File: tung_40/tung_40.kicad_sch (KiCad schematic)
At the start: 7 parts, among them J1 Conn_01x02_Male, J2 Conn_01x02_Male, SW1 GateronLP, SW5 SW_DIP_x03, U1 NRF52840-DONGLE

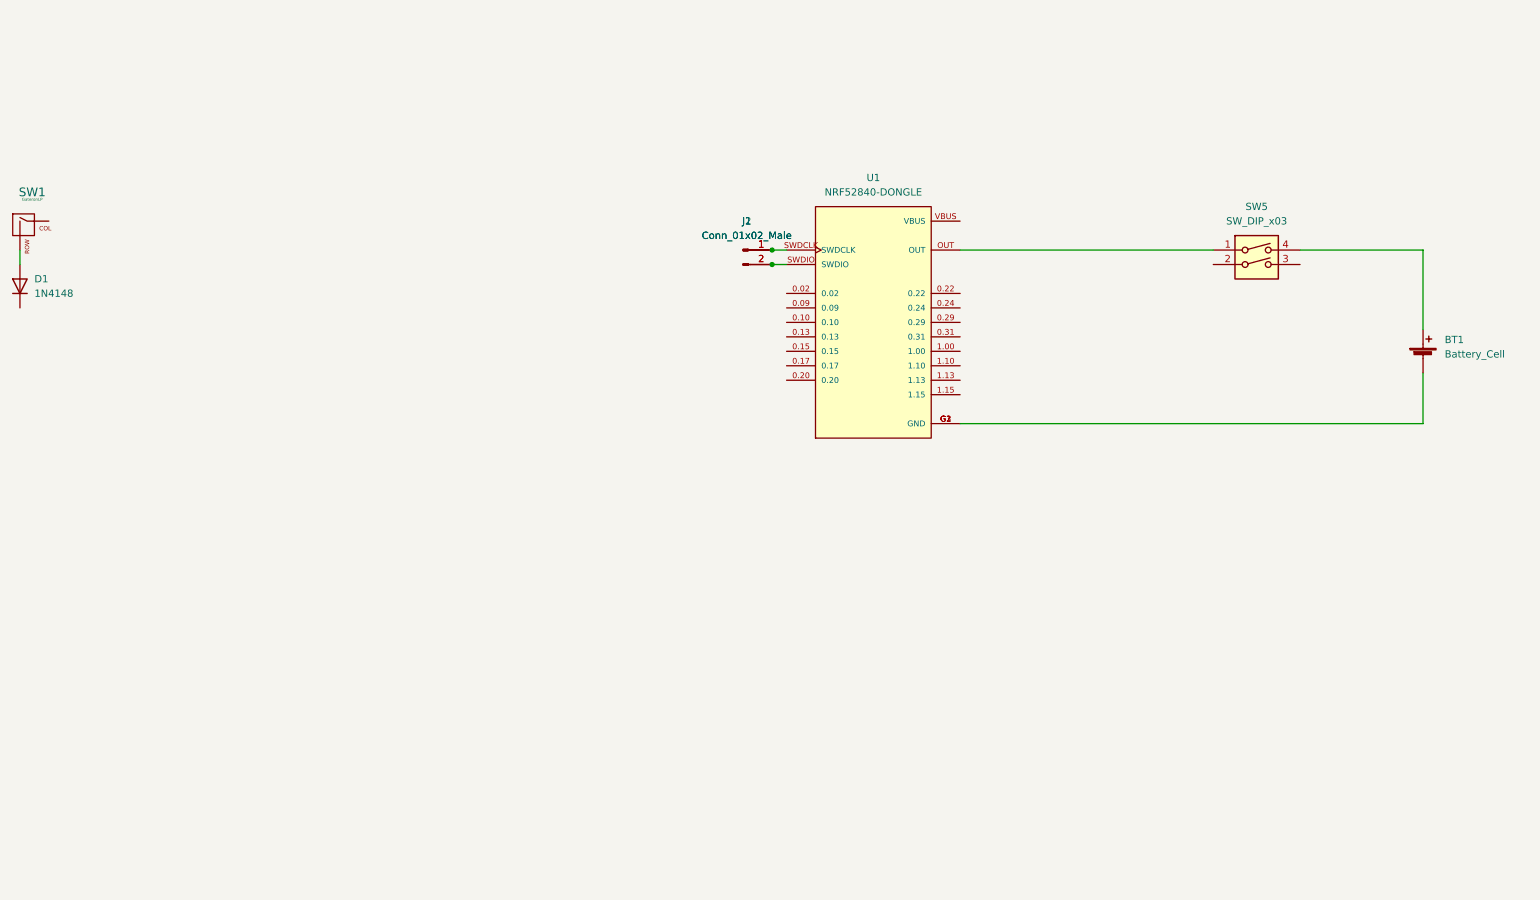
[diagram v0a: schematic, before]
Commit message: 48 keys in progress
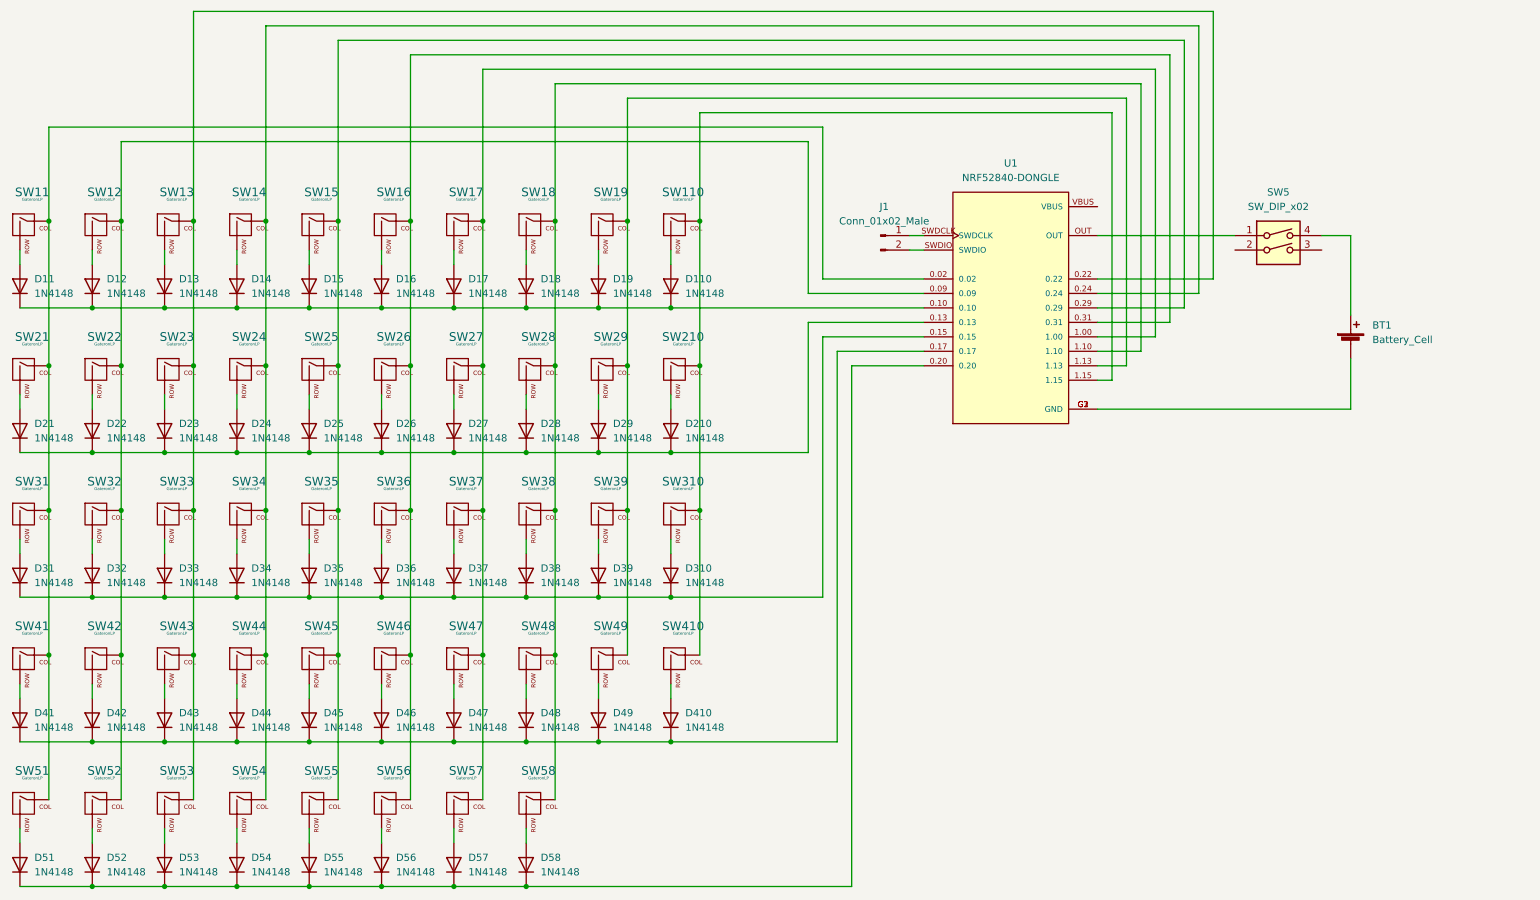
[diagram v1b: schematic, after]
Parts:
- removed J2: Conn_01x02_Male, Connector_PinHeader_2.54mm:PinHeader_1x02_P2.54mm_Vertical, symbol Connector:Conn_01x02_Male
- added D110, D12, D13, D14, D15, D16, D17, D18, D19, D21, D210, D22, D23, D24, D25, D26, D27, D28, D29, D31, D310, D32, D33, D34, D35, D36, D37, D38, D39, D41, D410, D42, D43, D44, D45, D46, D47, D48, D49, D51, D52, D53, D54, D55, D56, D57, D58: 1N4148, Diode_THT:D_DO-35_SOD27_P7.62mm_Horizontal, symbol Diode:1N4148
- added SW110, SW12, SW13, SW14, SW15, SW16, SW17, SW18, SW19, SW21, SW210, SW22, SW23, SW24, SW25, SW26, SW27, SW28, SW29, SW31, SW310, SW32, SW33, SW34, SW35, SW36, SW37, SW38, SW39, SW41, SW410, SW42, SW43, SW44, SW45, SW46, SW47, SW48, SW49, SW51, SW52, SW53, SW54, SW55, SW56, SW57, SW58: GateronLP, GateronLP:SW_Gateron_LO_PRO_1.00u_NO_LED_REVERSABLE_PCB, symbol GateronLP:GateronLP
- BT1: footprint Battery:Battery_Panasonic_CR2032-VS1N_Vertical_CircularHoles -> Misc:TBH-CR2032-M04
- SW11: renamed from SW1; footprint Button_Switch_Keyboard:SW_Cherry_MX_1.00u_PCB -> GateronLP:SW_Gateron_LO_PRO_1.00u_NO_LED_REVERSABLE_PCB; symbol gateronLowProfile:GateronLP -> GateronLP:GateronLP
- SW5: value SW_DIP_x03 -> SW_DIP_x02; footprint Button_Switch_THT:SW_DIP_SPSTx02_Slide_6.7x6.64mm_W7.62mm_P2.54mm_LowProfile -> Misc:SW_DIP_SPSTx02_Slide_9.78x7.26mm_W7.62mm_P2.54mm
- U1: footprint NRF52840-DONGLE:MODULE_NRF52840-DONGLE -> MODULE_NRF52840-DONGLE
- renumbered D1 to D11
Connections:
- net at SW11.1 (COL): now also U1.0.02, SW21.1 (COL), SW31.1 (COL), SW41.1 (COL), SW51.1 (COL)
- net at D11.1 (K): now also U1.0.10, D110.1 (K), D12.1 (K), D13.1 (K), D14.1 (K), D15.1 (K), D16.1 (K), D17.1 (K), D18.1 (K), D19.1 (K)
- net at U1.0.09: now also SW12.1 (COL), SW22.1 (COL), SW32.1 (COL), SW42.1 (COL), SW52.1 (COL)
- net at U1.0.13: now also D21.1 (K), D210.1 (K), D22.1 (K), D23.1 (K), D24.1 (K), D25.1 (K), D26.1 (K), D27.1 (K), D28.1 (K), D29.1 (K)
- net at U1.0.15: now also D31.1 (K), D310.1 (K), D32.1 (K), D33.1 (K), D34.1 (K), D35.1 (K), D36.1 (K), D37.1 (K), D38.1 (K), D39.1 (K)
- net at U1.0.17: now also D41.1 (K), D410.1 (K), D42.1 (K), D43.1 (K), D44.1 (K), D45.1 (K), D46.1 (K), D47.1 (K), D48.1 (K), D49.1 (K)
- net at U1.0.20: now also D51.1 (K), D52.1 (K), D53.1 (K), D54.1 (K), D55.1 (K), D56.1 (K), D57.1 (K), D58.1 (K)
- net at U1.0.22: now also SW13.1 (COL), SW23.1 (COL), SW33.1 (COL), SW43.1 (COL), SW53.1 (COL)
- net at U1.0.24: now also SW14.1 (COL), SW24.1 (COL), SW34.1 (COL), SW44.1 (COL), SW54.1 (COL)
- net at U1.0.29: now also SW15.1 (COL), SW25.1 (COL), SW35.1 (COL), SW45.1 (COL), SW55.1 (COL)
- net at U1.0.31: now also SW16.1 (COL), SW26.1 (COL), SW36.1 (COL), SW46.1 (COL), SW56.1 (COL)
- net at U1.1.00: now also SW17.1 (COL), SW27.1 (COL), SW37.1 (COL), SW47.1 (COL), SW57.1 (COL)
- net at U1.1.10: now also SW18.1 (COL), SW28.1 (COL), SW38.1 (COL), SW48.1 (COL), SW58.1 (COL)
- net at U1.1.13: now also SW19.1 (COL), SW29.1 (COL), SW39.1 (COL), SW49.1 (COL)
- net at U1.1.15: now also SW110.1 (COL), SW210.1 (COL), SW310.1 (COL), SW410.1 (COL)
- new net: D47.2 (A), SW47.2 (ROW)
- new net: D35.2 (A), SW35.2 (ROW)
- new net: D24.2 (A), SW24.2 (ROW)
- new net: D110.2 (A), SW110.2 (ROW)
- new net: D15.2 (A), SW15.2 (ROW)
- new net: D33.2 (A), SW33.2 (ROW)
- new net: D34.2 (A), SW34.2 (ROW)
- new net: D13.2 (A), SW13.2 (ROW)
- new net: D44.2 (A), SW44.2 (ROW)
- new net: D48.2 (A), SW48.2 (ROW)
- new net: D29.2 (A), SW29.2 (ROW)
- new net: D36.2 (A), SW36.2 (ROW)
- new net: D14.2 (A), SW14.2 (ROW)
- new net: D53.2 (A), SW53.2 (ROW)
- new net: D28.2 (A), SW28.2 (ROW)
- new net: D41.2 (A), SW41.2 (ROW)
- new net: D12.2 (A), SW12.2 (ROW)
- new net: D39.2 (A), SW39.2 (ROW)
- new net: D18.2 (A), SW18.2 (ROW)
- new net: D38.2 (A), SW38.2 (ROW)
- new net: D31.2 (A), SW31.2 (ROW)
- new net: D23.2 (A), SW23.2 (ROW)
- new net: D22.2 (A), SW22.2 (ROW)
- new net: D19.2 (A), SW19.2 (ROW)
- new net: D56.2 (A), SW56.2 (ROW)
- new net: D25.2 (A), SW25.2 (ROW)
- new net: D17.2 (A), SW17.2 (ROW)
- new net: D210.2 (A), SW210.2 (ROW)
- new net: D21.2 (A), SW21.2 (ROW)
- new net: D26.2 (A), SW26.2 (ROW)
- new net: D410.2 (A), SW410.2 (ROW)
- new net: D49.2 (A), SW49.2 (ROW)
- new net: D310.2 (A), SW310.2 (ROW)
- new net: D52.2 (A), SW52.2 (ROW)
- new net: D32.2 (A), SW32.2 (ROW)
- new net: D43.2 (A), SW43.2 (ROW)
- new net: D45.2 (A), SW45.2 (ROW)
- new net: D42.2 (A), SW42.2 (ROW)
- new net: D55.2 (A), SW55.2 (ROW)
- new net: D54.2 (A), SW54.2 (ROW)
- new net: D16.2 (A), SW16.2 (ROW)
- new net: D57.2 (A), SW57.2 (ROW)
- new net: D58.2 (A), SW58.2 (ROW)
- new net: D27.2 (A), SW27.2 (ROW)
- new net: D51.2 (A), SW51.2 (ROW)
- new net: D37.2 (A), SW37.2 (ROW)
- new net: D46.2 (A), SW46.2 (ROW)
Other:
- moved on the sheet: BT1, J1, SW5, U1
